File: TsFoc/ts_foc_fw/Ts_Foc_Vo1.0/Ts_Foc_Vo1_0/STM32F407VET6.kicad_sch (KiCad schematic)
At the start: 15 parts, among them SW2 BOTTOM, U3 STM32F407VET6, X1 25Mhz

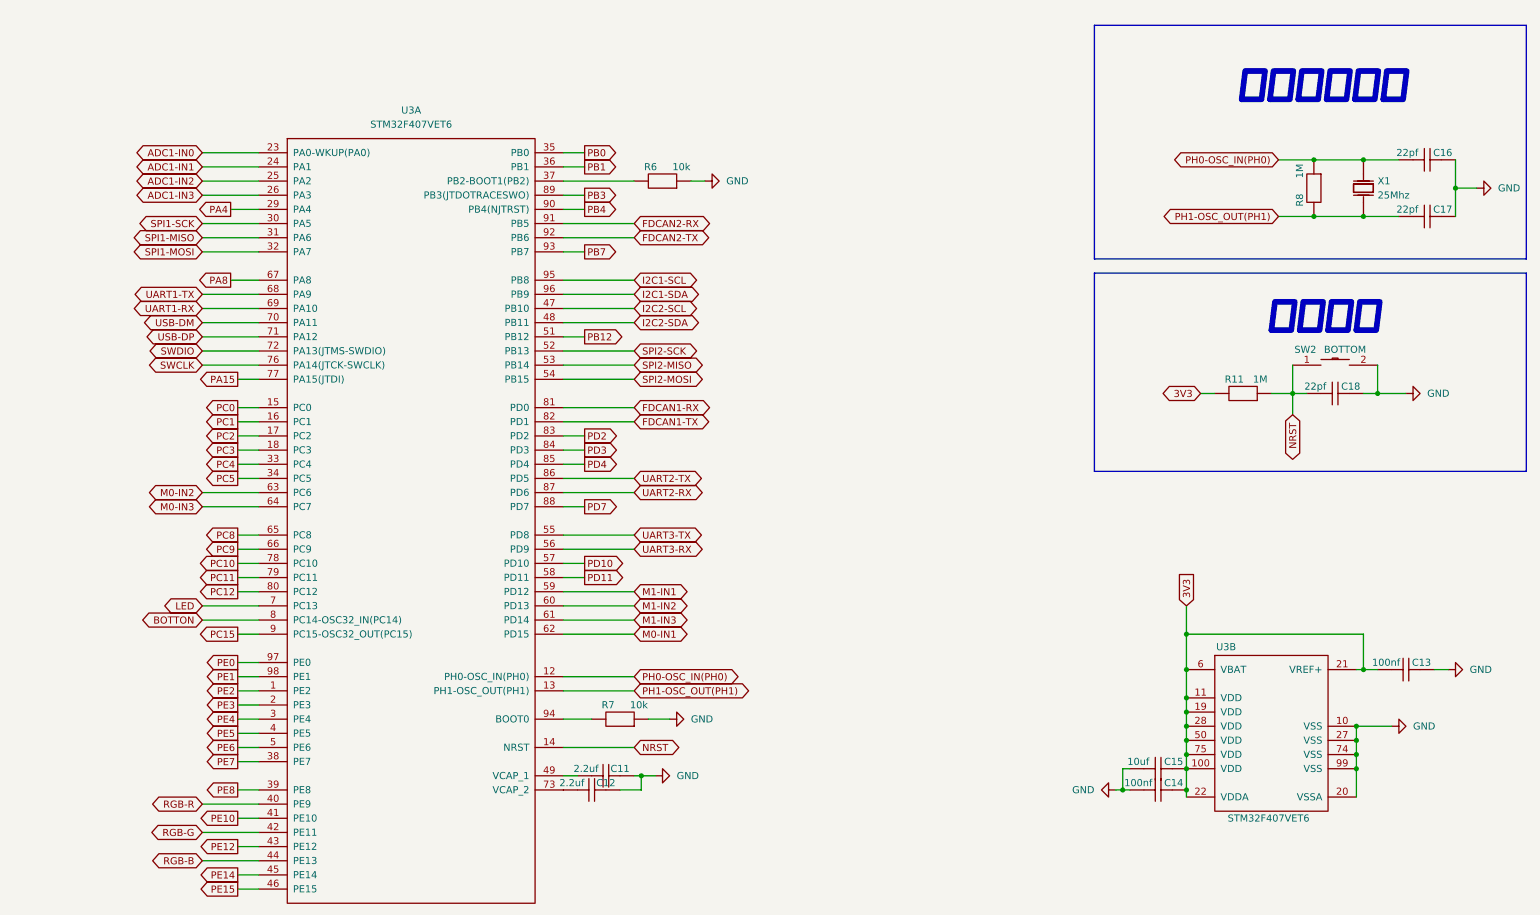
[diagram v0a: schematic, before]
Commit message: 同步_原理图小幅优化
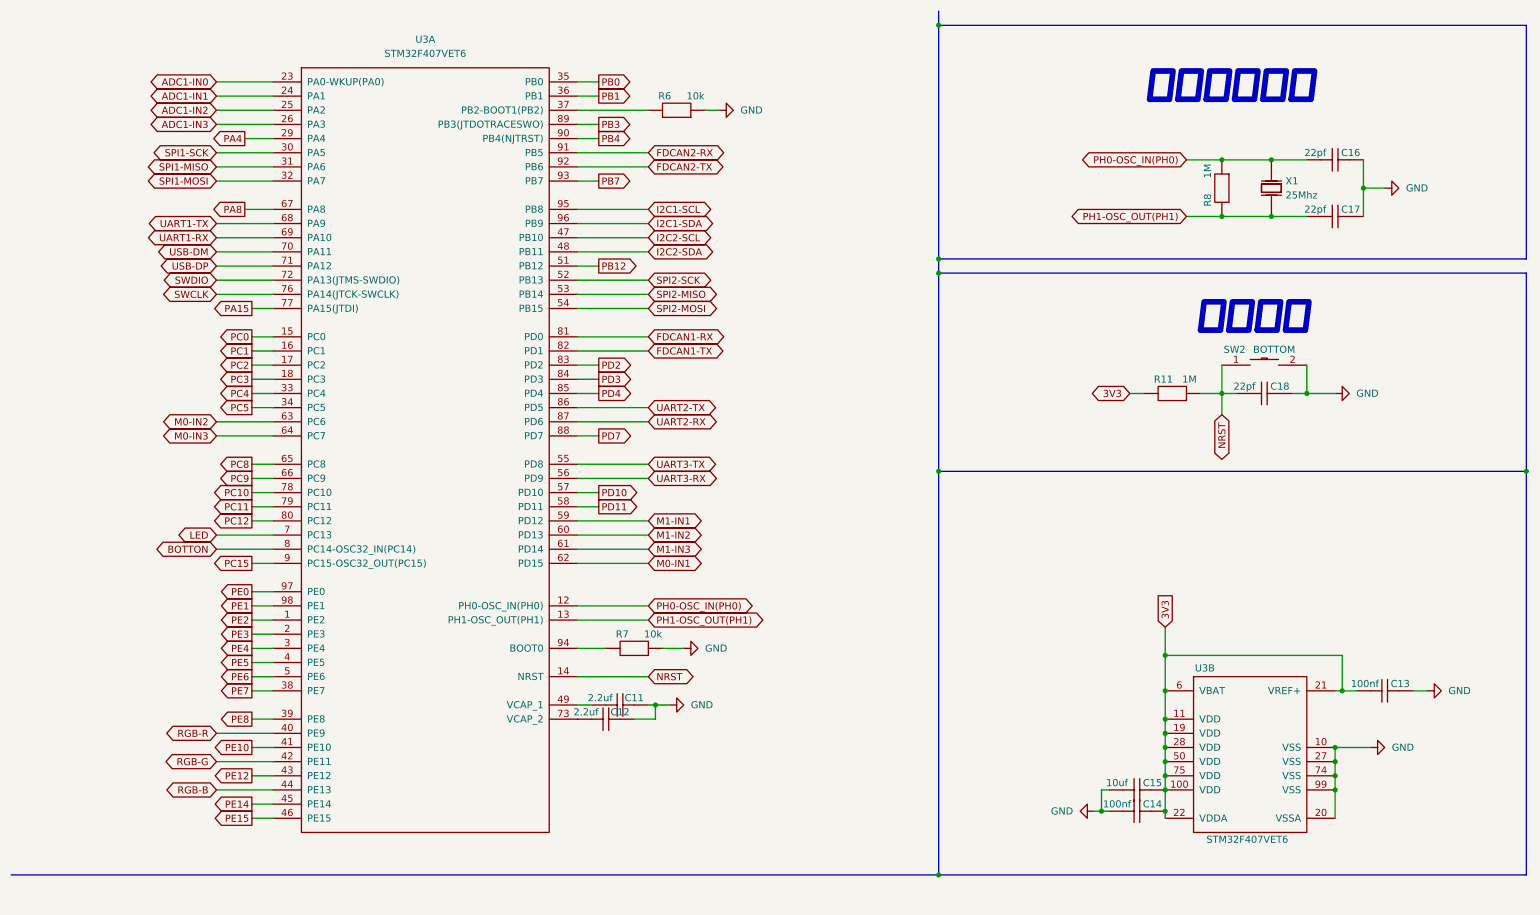
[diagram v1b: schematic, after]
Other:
- moved on the sheet: C11, C12, C13, C14, C15, C16, C17, C18, R11, R6, R7, R8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
